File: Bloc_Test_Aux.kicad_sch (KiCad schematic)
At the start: 45 parts, among them Q45 2N7000, Q46 2N7000, Q47 2N7000, Q48 2N7000, Q49 2N7000, Q50 2N7000

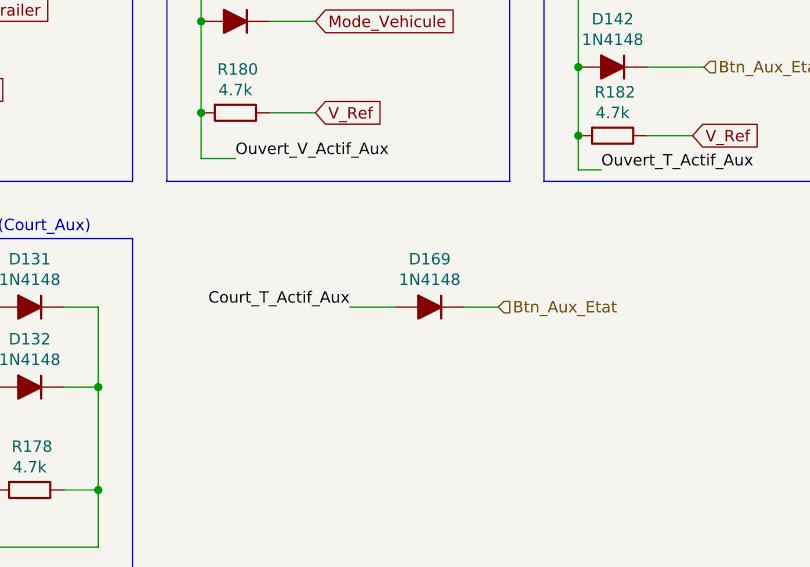
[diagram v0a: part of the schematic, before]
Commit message: Add files via upload
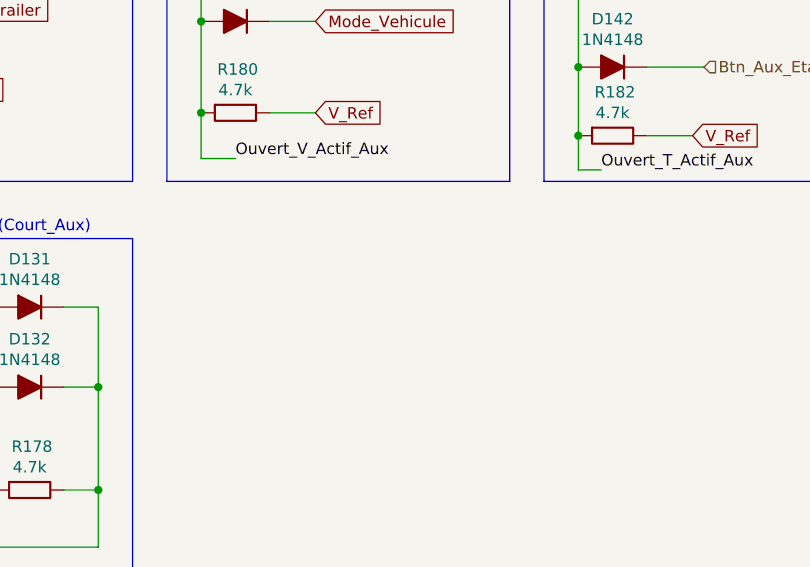
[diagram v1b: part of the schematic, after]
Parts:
- removed D169: 1N4148, PCM_Diode_THT_AKL:D_DO-35_SOD27_P7.62mm_Horizontal, symbol PCM_Diode_AKL:1N4148
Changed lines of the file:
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@@
 	(wire
 		(pts
-			(xy 123.19 80.01) (xy 128.27 80.01)
-		)
-		(stroke
-			(width 0)
-			(type default)
-		)
-	)
-	(wire
-		(pts
 			(xy 64.77 55.88) (xy 66.04 55.88)
 		)
@@
 	(wire
 		(pts
-			(xy 135.89 80.01) (xy 139.7 80.01)
-		)
-		(stroke
-			(width 0)
-			(type default)
-		)
-	)
-	(wire
-		(pts
 			(xy 114.3 58.42) (xy 119.38 58.42)
 		)
@@
 	)
 	(label "Court_T_Actif_Aux"
-		(at 123.19 80.01 180)
-		(effects
-			(font
-				(size 1.27 1.27)
-			)
-			(justify right bottom)
-		)
-	)
-	(label "Court_T_Actif_Aux"
 		(at 66.04 63.5 0)
 		(effects
@@
 	(hierarchical_label "Btn_Aux_Etat"
 		(shape input)
-		(at 139.7 80.01 0)
-		(effects
-			(font
-				(size 1.27 1.27)
-			)
-			(justify left)
-		)
-	)
-	(hierarchical_label "Btn_Aux_Etat"
-		(shape input)
 		(at 162.56 53.34 0)
 		(effects
@@
 					(unit 1)
 				)
-			)
-		)
-	)
-	(symbol
-		(lib_id "PCM_Diode_AKL:1N4148")
-		(at 132.08 80.01 0)
-		(unit 1)
-		(body_style 1)
-		(exclude_from_sim no)
-		(in_bom yes)
-		(on_board yes)
-		(in_pos_files yes)
-		(dnp no)
-		(property "Reference" "D169"
-			(at 132.08 74.676 0)
-			(show_name no)
-			(do_not_autoplace no)
-			(effects
-				(font
-					(size 1.27 1.27)
-				)
-			)
-		)
-		(property "Value" "1N4148"
-			(at 132.08 76.962 0)
-			(show_name no)
-			(do_not_autoplace no)
-			(effects
-				(font
-					(size 1.27 1.27)
-				)
-			)
-		)
-		(property "Footprint" "PCM_Diode_THT_AKL:D_DO-35_SOD27_P7.62mm_Horizontal"
-			(at 132.08 80.01 0)
-			(hide yes)
-			(show_name no)
-			(do_not_autoplace no)
-			(effects
-				(font
-					(size 1.27 1.27)
-				)
-			)
-		)
-		(property "Datasheet" "https://datasheet.octopart.com/1N4148TR-ON-Semiconductor-datasheet-42765246.pdf"
-			(at 132.08 80.01 0)
-			(hide yes)
-			(show_name no)
-			(do_not_autoplace no)
-			(effects
-				(font
-					(size 1.27 1.27)
-				)
-			)
-		)
-		(property "Description" "DO-35 Diode, Small Signal, Fast Switching, 75V, 150mA, 4ns, Alternate KiCad Library"
-			(at 132.08 80.01 0)
-			(hide yes)
-			(show_name no)
-			(do_not_autoplace no)
-			(effects
-				(font
-					(size 1.27 1.27)
-				)
-			)
-		)
-		(pin "2"
-		)
-		(pin "1"
-		)
-		(instances
-			(project "TrailerDiagnosticSystem"
-				(path "/d4e407a7-3e32-4226-ae57-831ecdb3edf4/f56287af-99ab-446e-8dde-0a4522148d74/d25077f7-2868-4779-a1c2-6faeaca9c2d4"
-					(reference "D169")
-					(unit 1)
-				)
